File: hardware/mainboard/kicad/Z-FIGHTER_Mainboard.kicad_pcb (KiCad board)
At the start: 2 copper layers, 100 x 150 mm, 55 parts, among them IC1 Z80SIO, J1 DB9_Male_MountingHoles, J2 DB9_Male_MountingHoles, J3 USB_B, J4 Conn_02x13_Odd_Even, J5 Conn_Parallel_User, J6 Conn_PATA, J7 Conn_02x04_Odd_Even, SW1 SW_Push, SW2 SW_DIP_x03, U1 AS6C4008-55PCN, U10 DS1233, U2 Z80CPU, U3 82C55A, U4 SST39SF040, U5 MAX203, U6 MAX203, U7 ATF22V10CZ-15PI, U8 74HC00, U9 82C55A, X1 Z80/SIO Ch.A Clock, X2 SIO Ch.B Clock

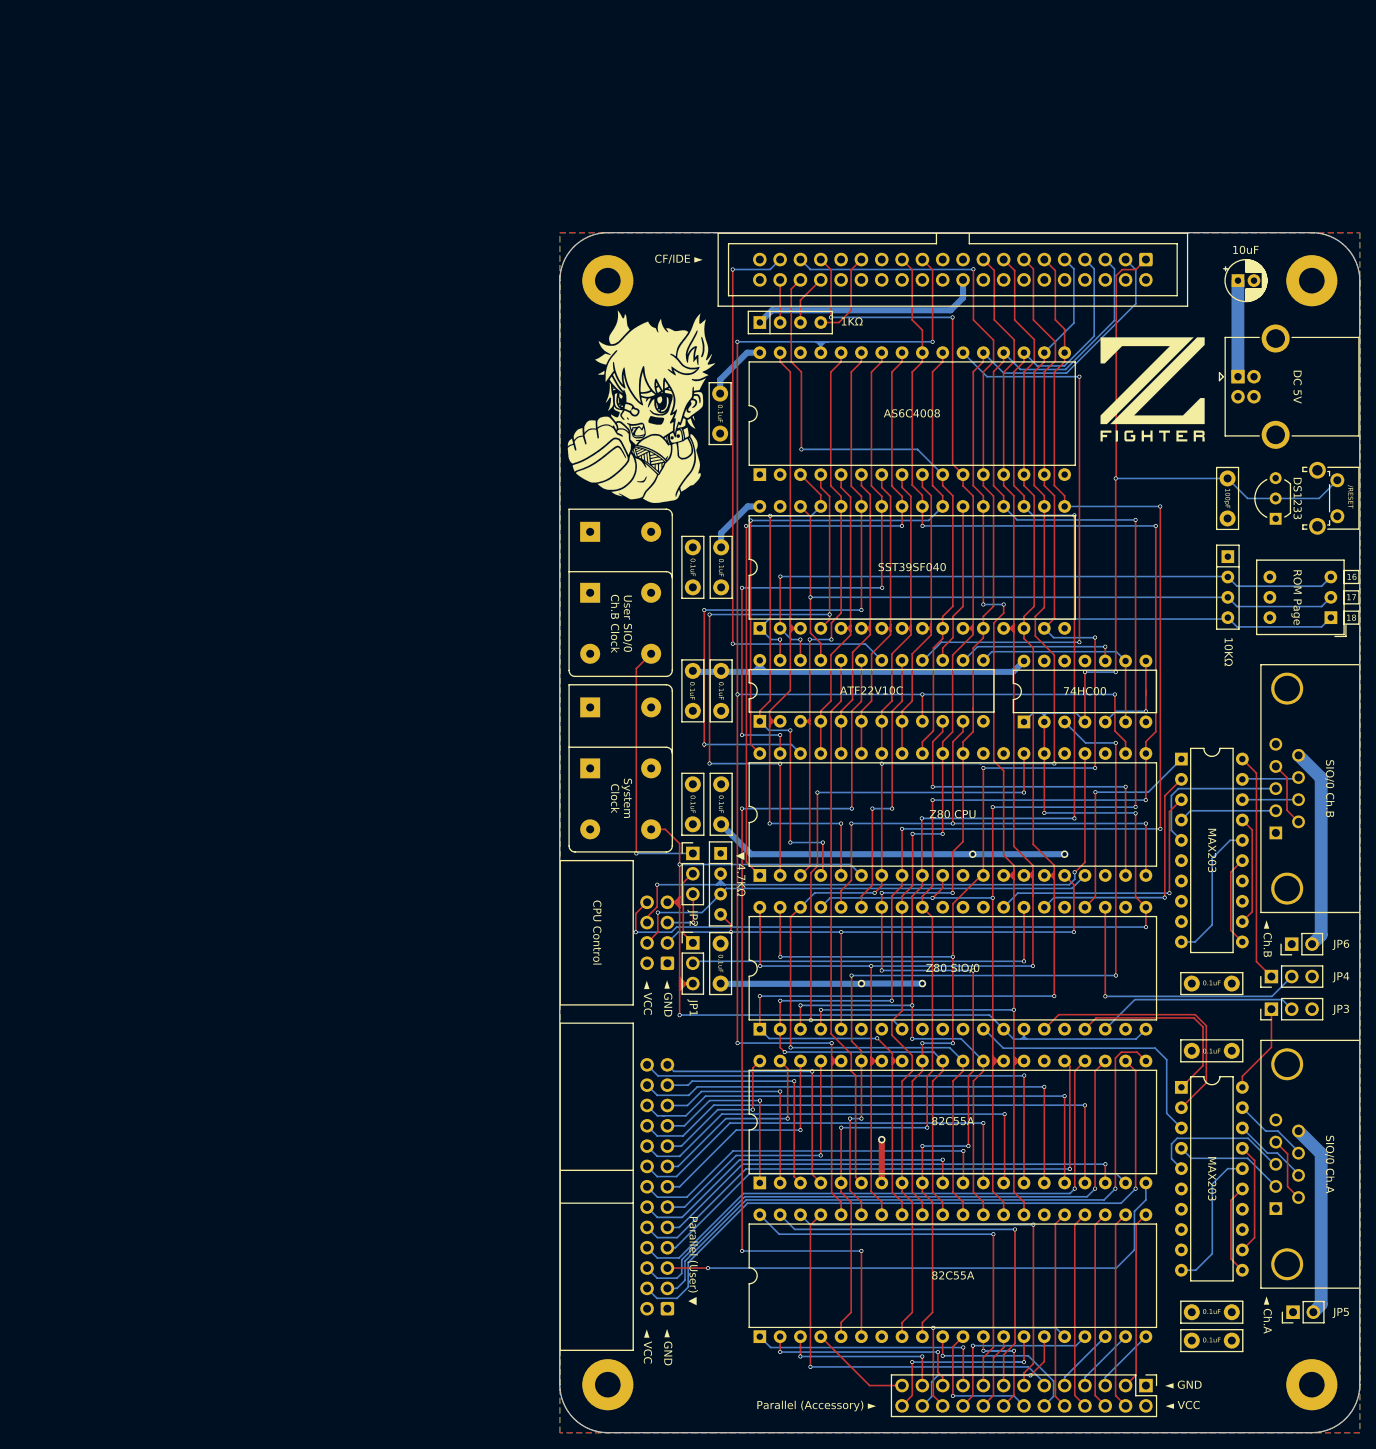
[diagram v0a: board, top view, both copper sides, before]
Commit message: Routing, plot, mainboard images
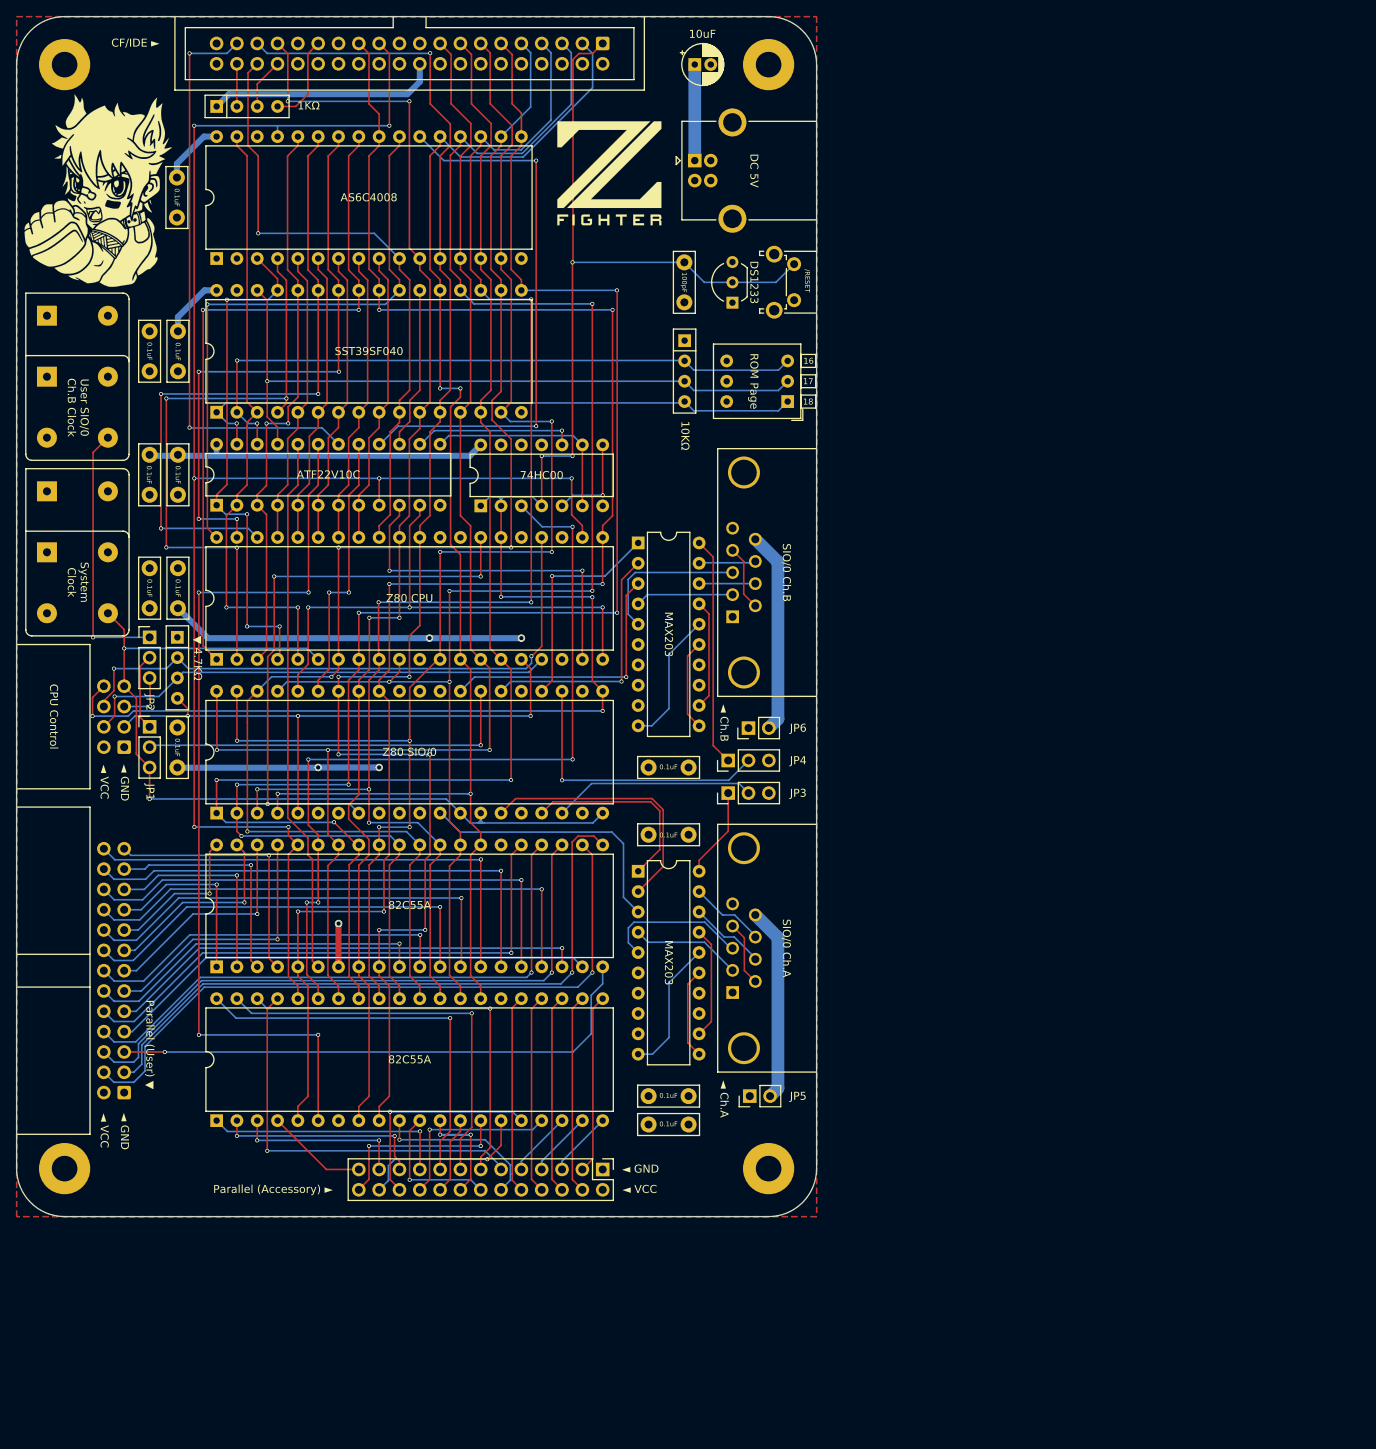
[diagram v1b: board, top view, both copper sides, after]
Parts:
- moved C10 73.1 mm to (79.0, 134.9)
- moved C12 73.1 mm to (79.0, 93.9)
- moved C13 73.1 mm to (84.0, 102.3)
- moved C14 73.1 mm to (16.6, 39.3)
- moved C2 73.1 mm to (83.5, 35.7)
- moved C3 73.1 mm to (16.6, 69.0)
- moved C4 73.1 mm to (20.0, 20.1)
- moved C5 73.1 mm to (79.0, 138.5)
- moved C9 73.1 mm to (16.6, 54.8)
- moved J1 73.1 mm to (89.5, 122.0)
- moved J2 73.1 mm to (89.5, 75.0)
- moved JP1 73.1 mm to (16.6, 88.8)
- moved JP2 73.1 mm to (16.6, 77.6)
- moved JP6 73.1 mm to (91.5, 88.9)
- moved Mount2 73.1 mm to (94.0, 6.00)
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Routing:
- net CLOCK: track 129.0 -> 112.6 mm
- net D0: track 183.3 -> 167.2 mm
- net D7: track 182.5 -> 170.8 mm
- net #WR: track 225.8 -> 217.3 mm
- net D1: track 185.7 -> 177.3 mm
- net A15: track 85.0 -> 77.0 mm
- net A7: track 41.6 -> 36.9 mm
- net #WAIT: track 79.1 -> 74.5 mm
- net D6: track 199.2 -> 194.5 mm
- net A6: track 41.4 -> 36.8 mm
- net A1: track 164.2 -> 160.8 mm
- net A5: track 40.0 -> 36.8 mm
- net A3: track 40.0 -> 36.8 mm
- net A4: track 39.9 -> 36.8 mm
- net VCC: track 173.3 -> 170.3 mm
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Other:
- net class Default removed
- net class Power removed
